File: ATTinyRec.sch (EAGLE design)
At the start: 13 parts, among them M1 ELECTRET_MICROPHON-WM-62PC/62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, U2 USD-SOCKETUSD

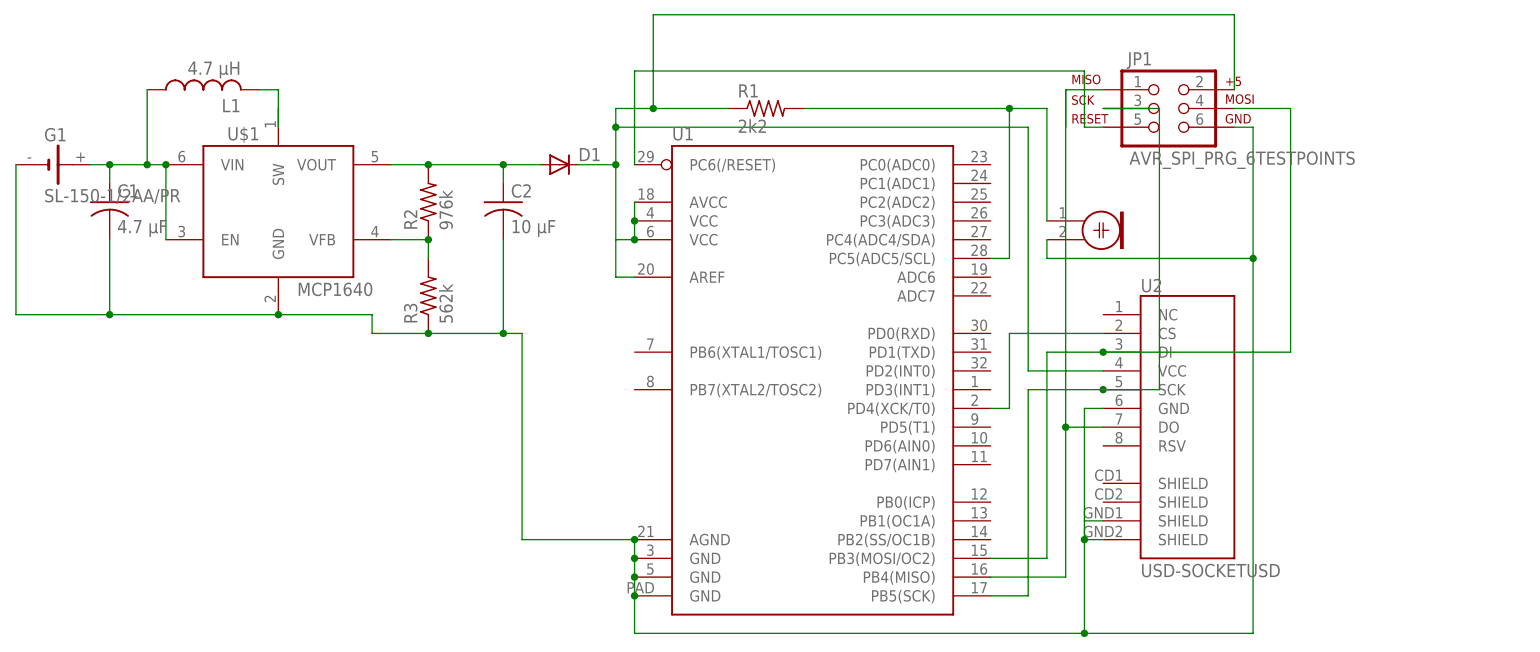
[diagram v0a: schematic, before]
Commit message: Routed
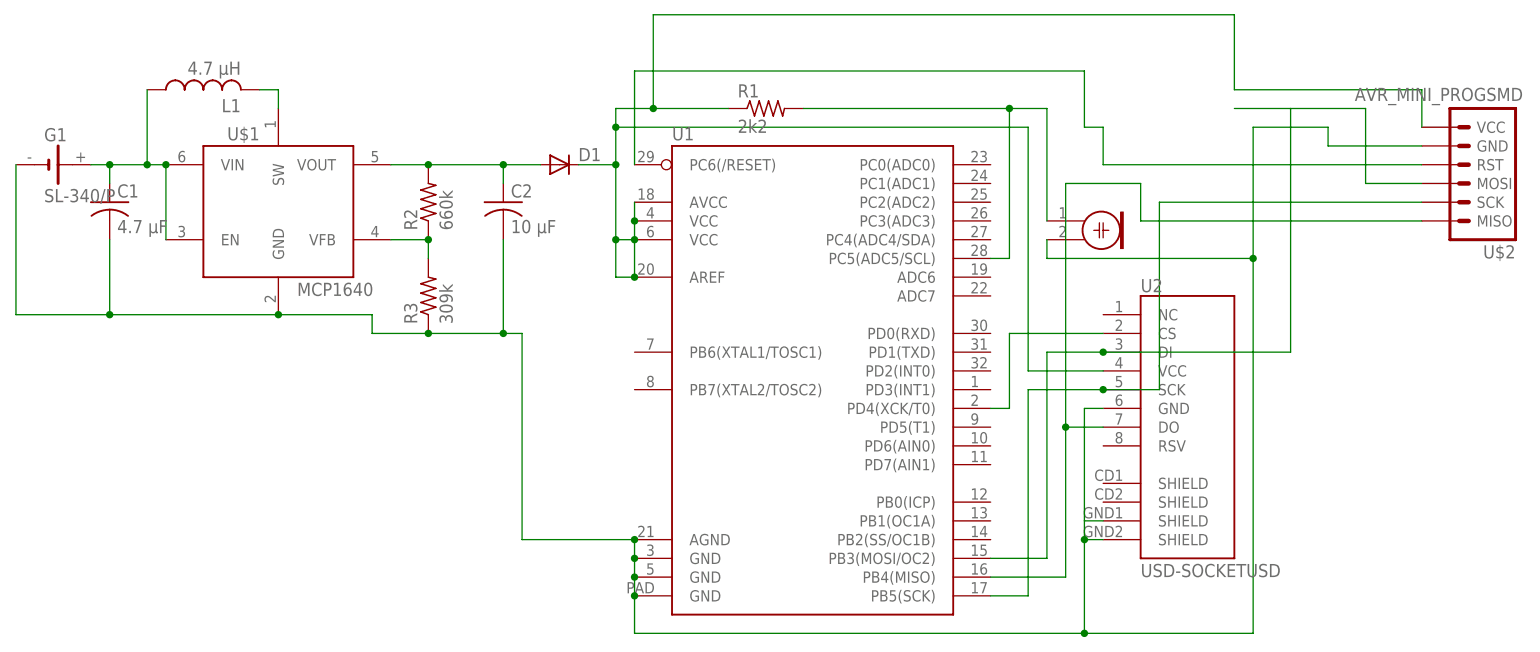
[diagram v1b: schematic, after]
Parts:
- removed JP1: AVR_SPI_PRG_6TESTPOINTS, SparkFun-Connectors:AVR_SPI_PRG_6TESTPOINTS
- added U$2: AVR_MINI_PROGSMD, SparkFun-Connectors:AVR_MINI_PROGSMD
- C1, C2: device rcl:C-USC0805K -> rcl:C-USC0402
- G1: value SL-150-1/2AA/PR -> SL-340/P; device battery:SL-150-1/2AA/PR -> battery:SL-340/P
- L1: device rcl:L-USL2825P -> resistor:L-USL2012C
- R1: device resistor:R-US_M0805 -> rcl:R-US_R0402
- R2: value 976k -> 660k; device resistor:R-US_M0805 -> rcl:R-US_R0402
- R3: value 562k -> 309k; device resistor:R-US_M0805 -> rcl:R-US_R0402
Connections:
- removed net N$5: D1.C, JP1.2, R1.1, U1.AREF, U2.VCC
- net N$20: now also U$2.RST; no longer JP1.5
- net N$3: now also U$1.SW
- net N$4: now also U$2.GND; no longer JP1.6
- net N$6: now also U$2.MOSI; no longer JP1.4
- net N$7: now also U$2.MISO; no longer JP1.1
- net N$9: now also U$2.SCK; no longer JP1.3
- net NET': now also D1.C, R1.1, U$2.VCC, U1.AREF, U2.VCC
